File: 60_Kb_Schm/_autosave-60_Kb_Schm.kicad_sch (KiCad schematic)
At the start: 2 parts

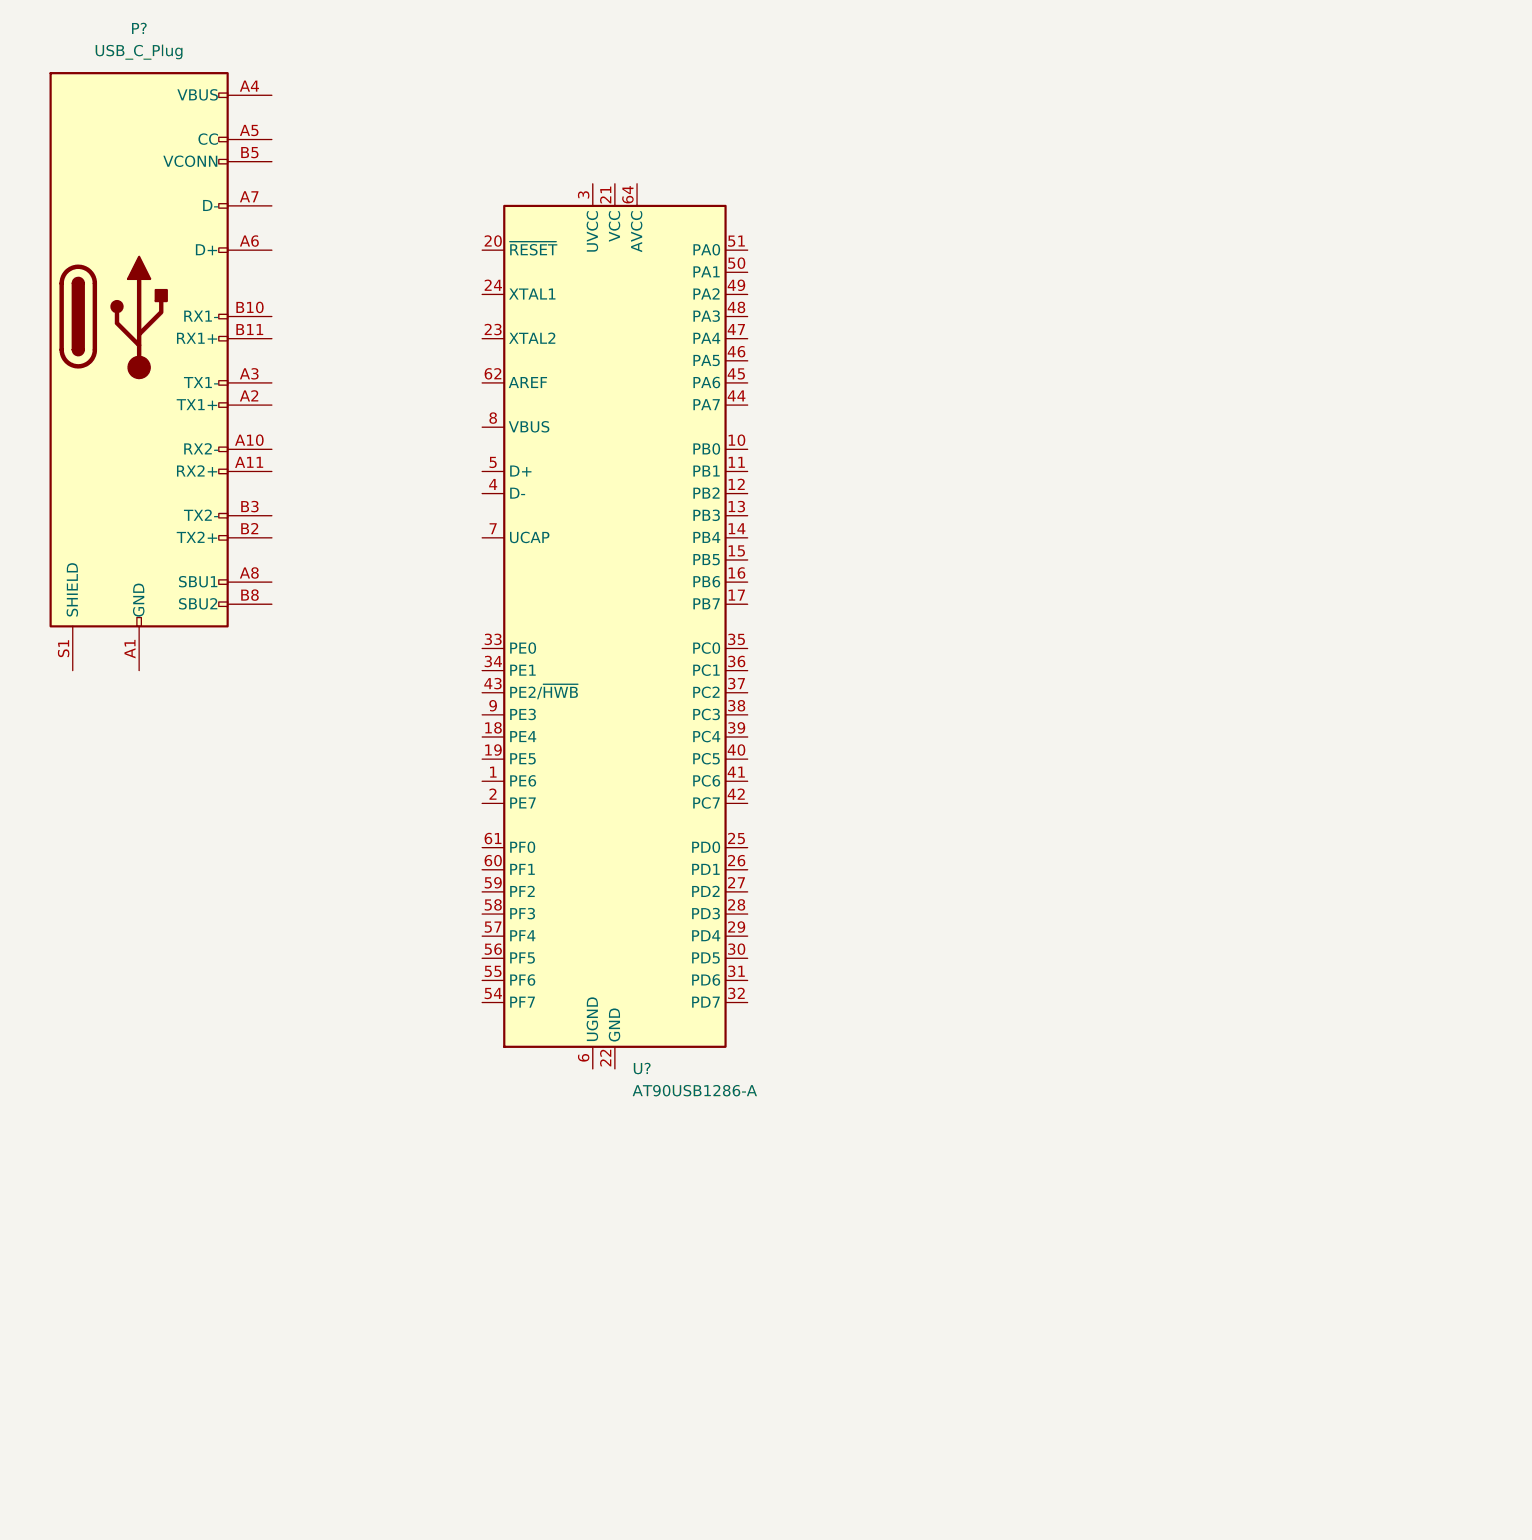
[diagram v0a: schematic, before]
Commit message: update
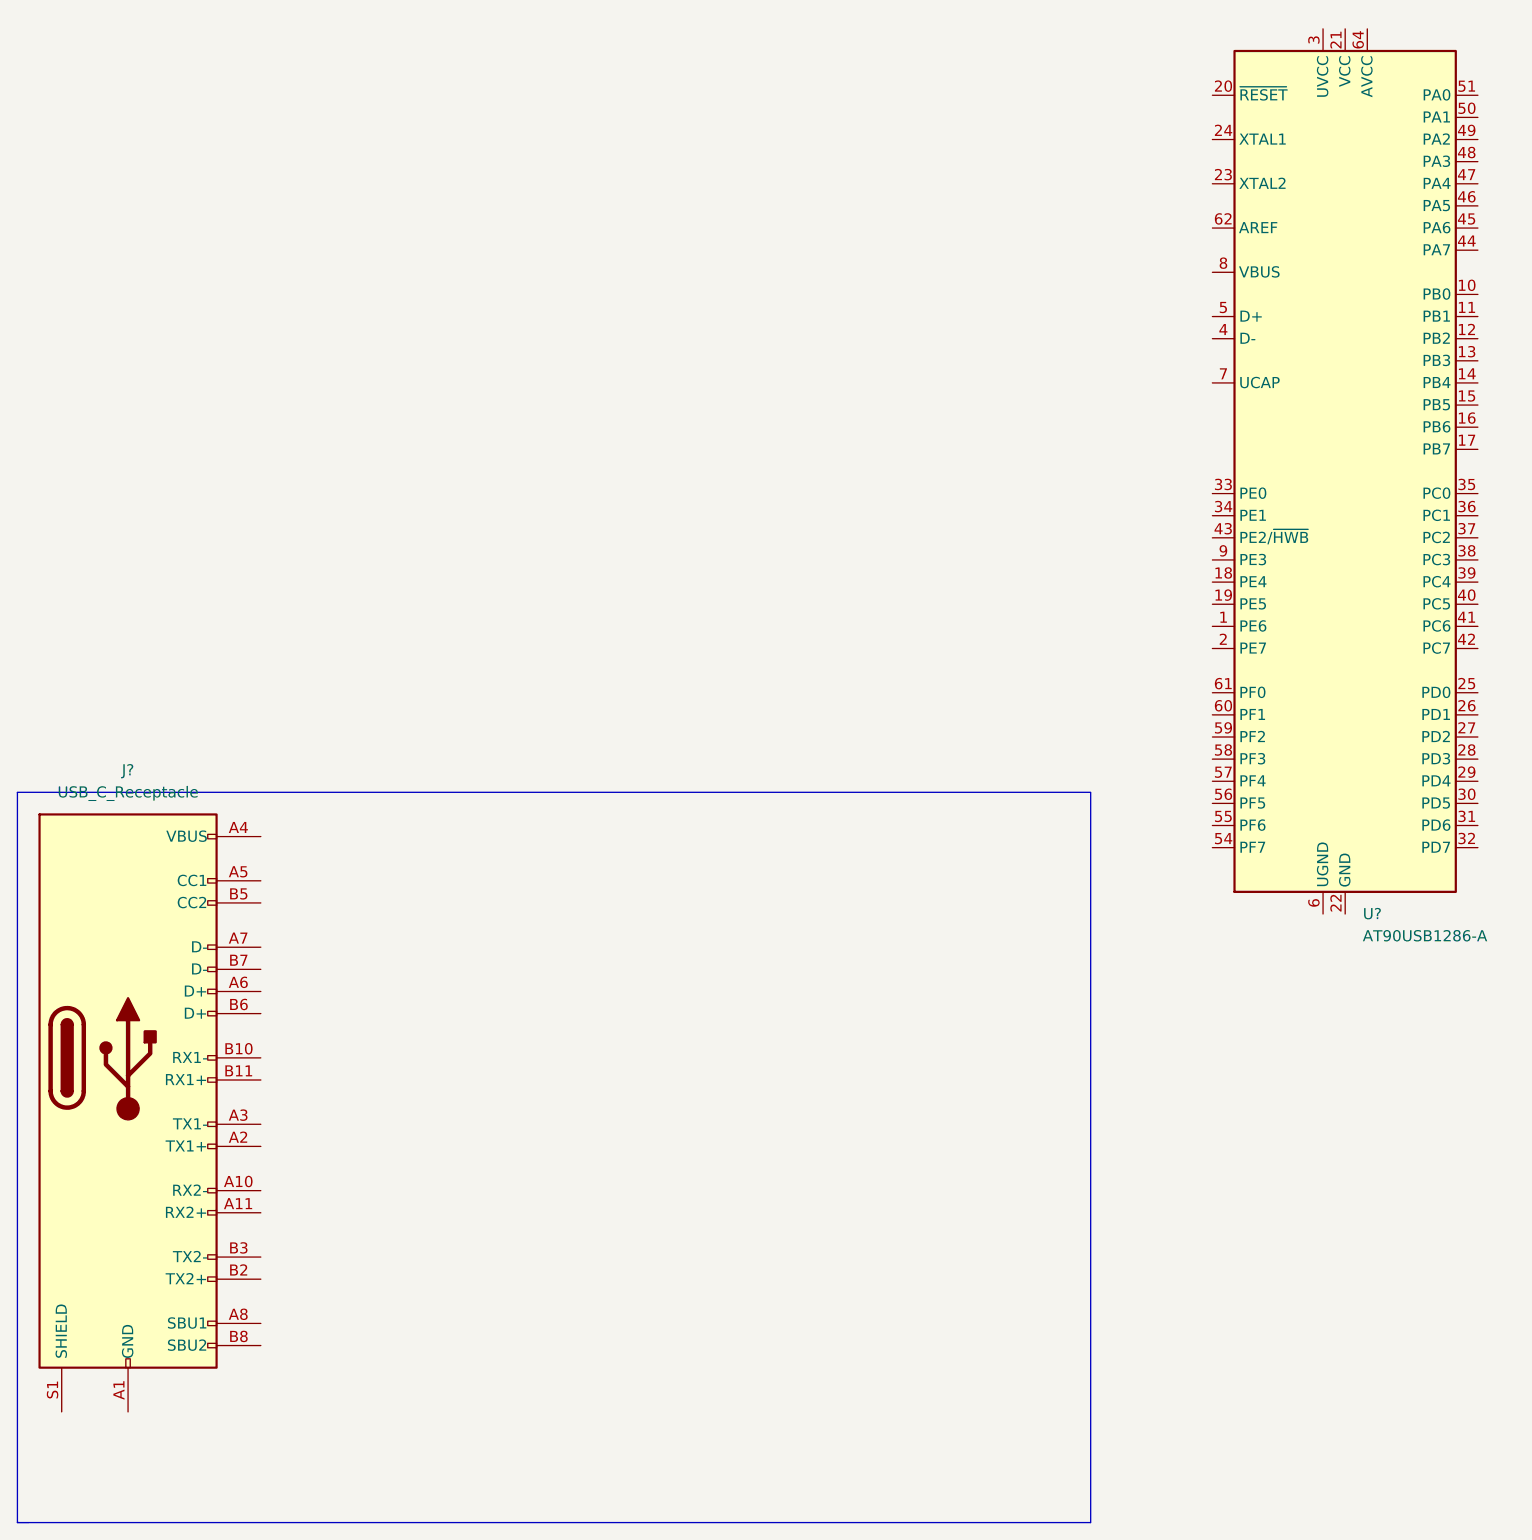
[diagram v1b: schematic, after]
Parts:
- removed P?: USB_C_Plug, symbol Connector:USB_C_Plug
- added J?: USB_C_Receptacle, symbol Connector:USB_C_Receptacle
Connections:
- new net: J?.A1 (GND), J?.A12 (GND), J?.B1 (GND), J?.B12 (GND)
- new net: J?.A4 (VBUS), J?.A9 (VBUS), J?.B4 (VBUS), J?.B9 (VBUS)
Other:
- moved on the sheet: U?
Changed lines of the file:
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@@
 (kicad_sch (version 20211123) (generator eeschema)
   (paper "A4")
-  (symbol (lib_id "MCU_Microchip_AVR:AT90USB1286-A") (at 82.55 91.44 0) (unit 1)
+  (polyline (pts (xy 13.97 110.49) (xy 13.97 194.31))
+    (stroke (width 0) (type default) (color 0 0 0 0))
+  )
+  (polyline (pts (xy 137.16 110.49) (xy 137.16 194.31))
+    (stroke (width 0) (type default) (color 0 0 0 0))
+  )
+  (polyline (pts (xy 13.97 110.49) (xy 137.16 110.49))
+    (stroke (width 0) (type default) (color 0 0 0 0))
+  )
+  (polyline (pts (xy 137.16 194.31) (xy 13.97 194.31))
+    (stroke (width 0) (type default) (color 0 0 0 0))
+  )
+  (polyline (pts (xy 13.97 194.31) (xy 15.24 194.31))
+    (stroke (width 0) (type default) (color 0 0 0 0))
+  )
+  (symbol (lib_id "Connector:USB_C_Receptacle") (at 26.67 140.97 0) (unit 1)
     (in_bom yes) (on_board yes) (fields_autoplaced)
-    (property "Reference" "U?" (id 0) (at 84.5694 142.24 0)
+    (property "Reference" "J?" (id 0) (at 26.67 107.95 0))
+    (property "Value" "USB_C_Receptacle" (id 1) (at 26.67 110.49 0))
+    (property "Footprint" "" (id 2) (at 30.48 140.97 0)
+      (effects (font (size 1.27 1.27)) hide)
+    )
+    (property "Datasheet" "https://www.usb.org/sites/default/files/documents/usb_type-c.zip" (id 3) (at 30.48 140.97 0)
+      (effects (font (size 1.27 1.27)) hide)
+    )
+    (pin "A1")
+    (pin "A10")
+    (pin "A11")
+    (pin "A12")
+    (pin "A2")
+    (pin "A3")
+    (pin "A4")
+    (pin "A5")
+    (pin "A6")
+    (pin "A7")
+    (pin "A8")
+    (pin "A9")
+    (pin "B1")
+    (pin "B10")
+    (pin "B11")
+    (pin "B12")
+    (pin "B2")
+    (pin "B3")
+    (pin "B4")
+    (pin "B5")
+    (pin "B6")
+    (pin "B7")
+    (pin "B8")
+    (pin "B9")
+    (pin "S1")
+  )
+  (symbol (lib_id "MCU_Microchip_AVR:AT90USB1286-A") (at 166.37 73.66 0) (unit 1)
+    (in_bom yes) (on_board yes) (fields_autoplaced)
+    (property "Reference" "U?" (id 0) (at 168.3894 124.46 0)
       (effects (font (size 1.27 1.27)) (justify left))
     )
-    (property "Value" "AT90USB1286-A" (id 1) (at 84.5694 144.78 0)
+    (property "Value" "AT90USB1286-A" (id 1) (at 168.3894 127 0)
       (effects (font (size 1.27 1.27)) (justify left))
     )
-    (property "Footprint" "Package_QFP:TQFP-64_14x14mm_P0.8mm" (id 2) (at 82.55 91.44 0)
+    (property "Footprint" "Package_QFP:TQFP-64_14x14mm_P0.8mm" (id 2) (at 166.37 73.66 0)
       (effects (font (size 1.27 1.27) italic) hide)
     )
-    (property "Datasheet" "http://ww1.microchip.com/downloads/en/DeviceDoc/doc7593.pdf" (id 3) (at 82.55 91.44 0)
+    (property "Datasheet" "http://ww1.microchip.com/downloads/en/DeviceDoc/doc7593.pdf" (id 3) (at 166.37 73.66 0)
       (effects (font (size 1.27 1.27)) hide)
     )
@@
     (pin "9")
   )
-  (symbol (lib_id "Connector:USB_C_Plug") (at 27.94 55.88 0) (unit 1)
-    (in_bom yes) (on_board yes) (fields_autoplaced)
-    (property "Reference" "P?" (id 0) (at 27.94 22.86 0))
-    (property "Value" "USB_C_Plug" (id 1) (at 27.94 25.4 0))
-    (property "Footprint" "" (id 2) (at 31.75 55.88 0)
-      (effects (font (size 1.27 1.27)) hide)
-    )
-    (property "Datasheet" "https://www.usb.org/sites/default/files/documents/usb_type-c.zip" (id 3) (at 31.75 55.88 0)
-      (effects (font (size 1.27 1.27)) hide)
-    )
-    (pin "A1")
-    (pin "A10")
-    (pin "A11")
-    (pin "A12")
-    (pin "A2")
-    (pin "A3")
-    (pin "A4")
-    (pin "A5")
-    (pin "A6")
-    (pin "A7")
-    (pin "A8")
-    (pin "A9")
-    (pin "B1")
-    (pin "B10")
-    (pin "B11")
-    (pin "B12")
-    (pin "B2")
-    (pin "B3")
-    (pin "B4")
-    (pin "B5")
-    (pin "B8")
-    (pin "B9")
-    (pin "S1")
-  )
   (sheet_instances
     (path "/" (page "1"))
   )
   (symbol_instances
-    (path "/a545b107-7c6a-4540-b695-807d3c10cd4f"
-      (reference "P?") (unit 1) (value "USB_C_Plug") (footprint "")
+    (path "/6572bce5-fced-4d2a-a775-b48b15573466"
+      (reference "J?") (unit 1) (value "USB_C_Receptacle") (footprint "")
     )
     (path "/8a2b6611-069e-4c89-9128-394138c65954"
